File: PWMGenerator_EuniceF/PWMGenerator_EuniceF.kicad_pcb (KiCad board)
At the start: 2 copper layers, 30 parts, among them J1 Conn_01x03_Pin, J2 Barrel_Jack, Q1 Q_PNP_BCE, Q3 2N3904, Q4 Q_PNP_BCE, Q7 2N3904, SW1 SW_SPST, U1 LM7805_TO220, U2 LM339

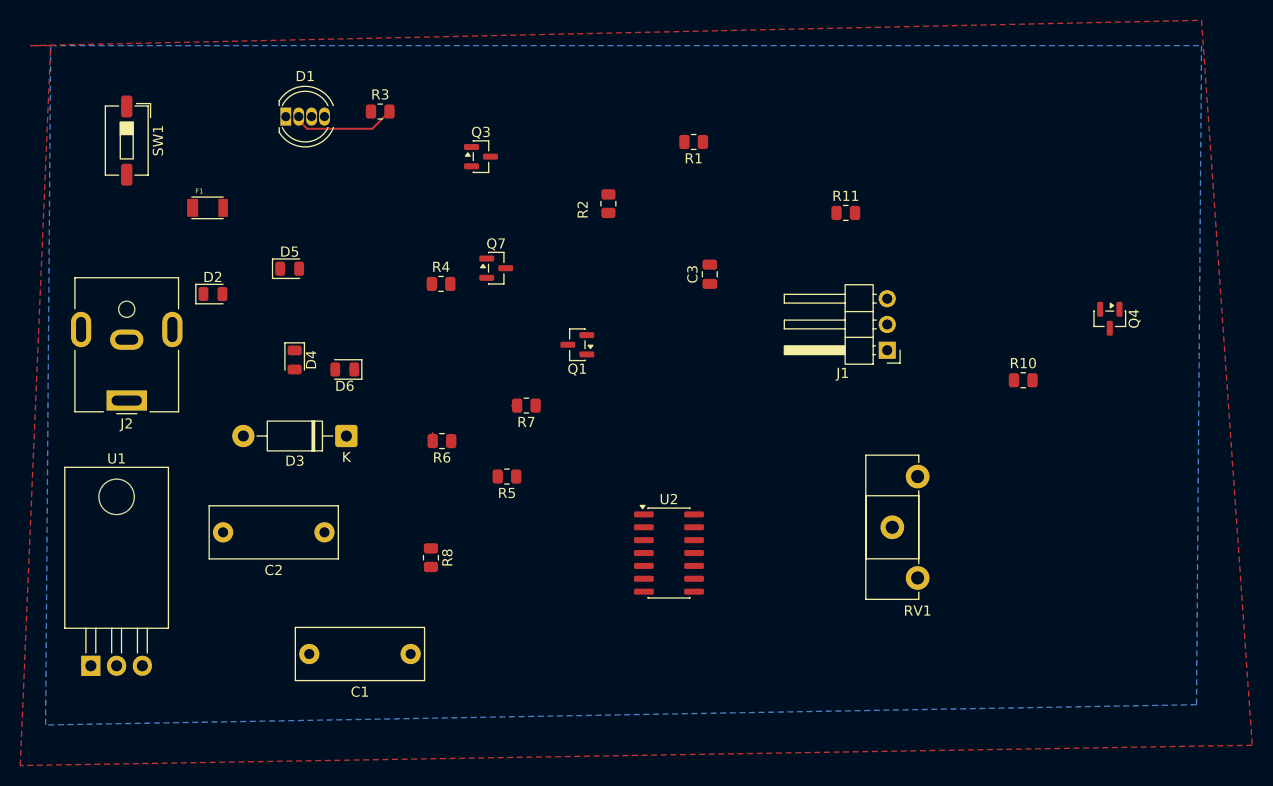
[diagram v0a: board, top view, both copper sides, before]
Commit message: PCB PARTC WORKING
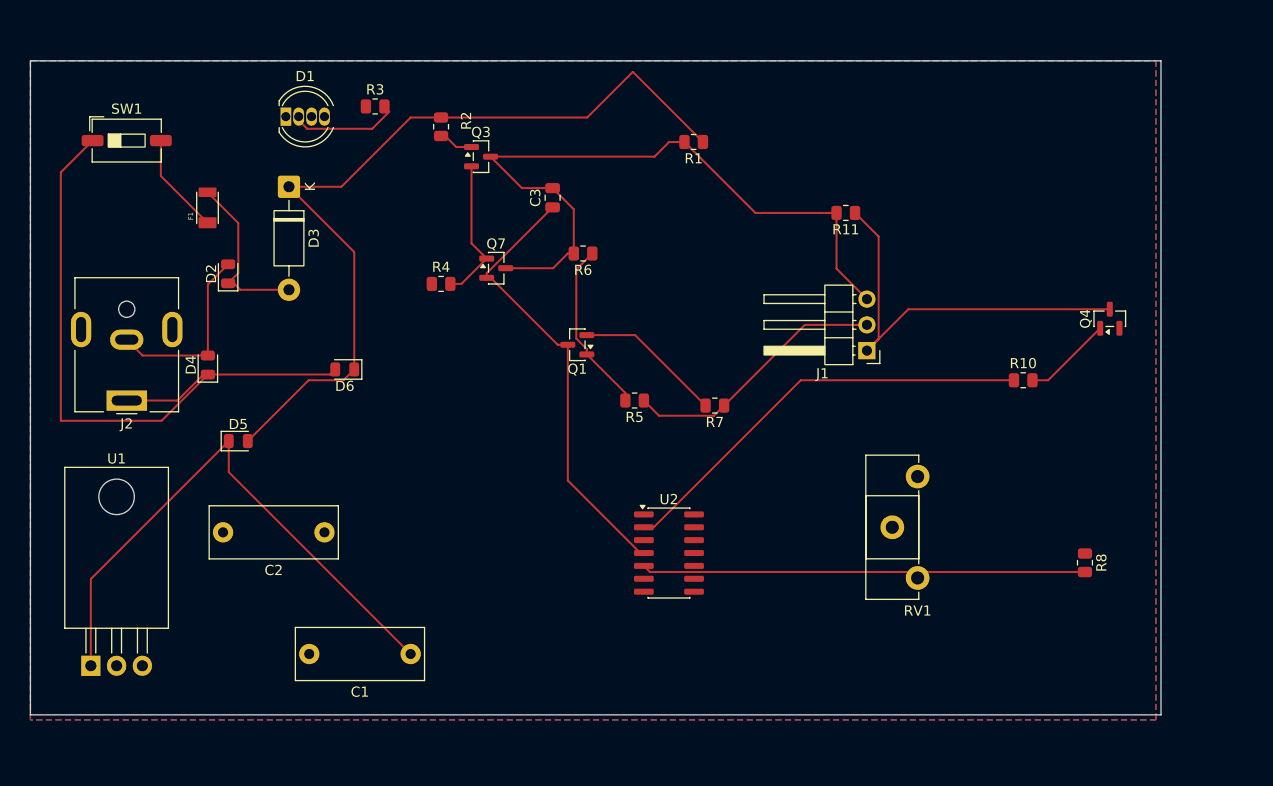
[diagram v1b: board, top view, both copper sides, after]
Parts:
- moved R8 64.5 mm to (119.0, 109.5)
- moved D3 25.2 mm to (40.5, 72.4), turned to -90 degrees
- moved R6 23.1 mm to (69.5, 79.0)
- moved R7 18.6 mm to (82.5, 94.0)
- moved R2 18.2 mm to (55.5, 66.5), turned to -90 degrees
- moved D5 17.7 mm to (35.5, 97.5)
- moved C3 17.2 mm to (66.5, 73.5)
- moved R5 14.7 mm to (74.6, 93.5)
- moved D4 8.58 mm to (32.5, 90.0), turned to 90 degrees
- moved D2 2.50 mm to (34.5, 81.0), turned to 90 degrees
- moved J1 2.00 mm to (97.5, 88.6)
- moved R3 0.71 mm to (49.0, 64.5)
- turned F1 to 90 degrees
- turned Q4 to 90 degrees
- turned R11 to 180 degrees
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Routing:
- net GND: track 1.28 -> 87.9 mm
- net Net-(D3-K): track 1.10 -> 82.5 mm
- net Net-(D4-K): track 0.00 -> 67.2 mm
- net Net-(D5-K): track 0.00 -> 56.2 mm
- net Net-(U2A-+): track 0.00 -> 44.2 mm
- net Net-(Q1-E): track 0.00 -> 44.2 mm
- net Net-(R10-Pad1): track 0.00 -> 42.5 mm
- net PWM: track 0.00 -> 40.3 mm
- net VCC 5V: track 0.00 -> 26.3 mm
- net Net-(D2-K): track 0.01 -> 17.8 mm
- net Net-(Q1-B): track 0.50 -> 17.2 mm
- net Net-(Q3-C): track 0.00 -> 14.3 mm
- net Net-(Q1-C): track 0.50 -> 14.6 mm
- net Net-(SW1-B): track 0.00 -> 10.0 mm
- net Net-(Q4-B): track 0.00 -> 8.80 mm
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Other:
- board outline added: 111.5 x 64.5 mm
